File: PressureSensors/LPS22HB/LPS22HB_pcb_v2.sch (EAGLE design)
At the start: 6 parts

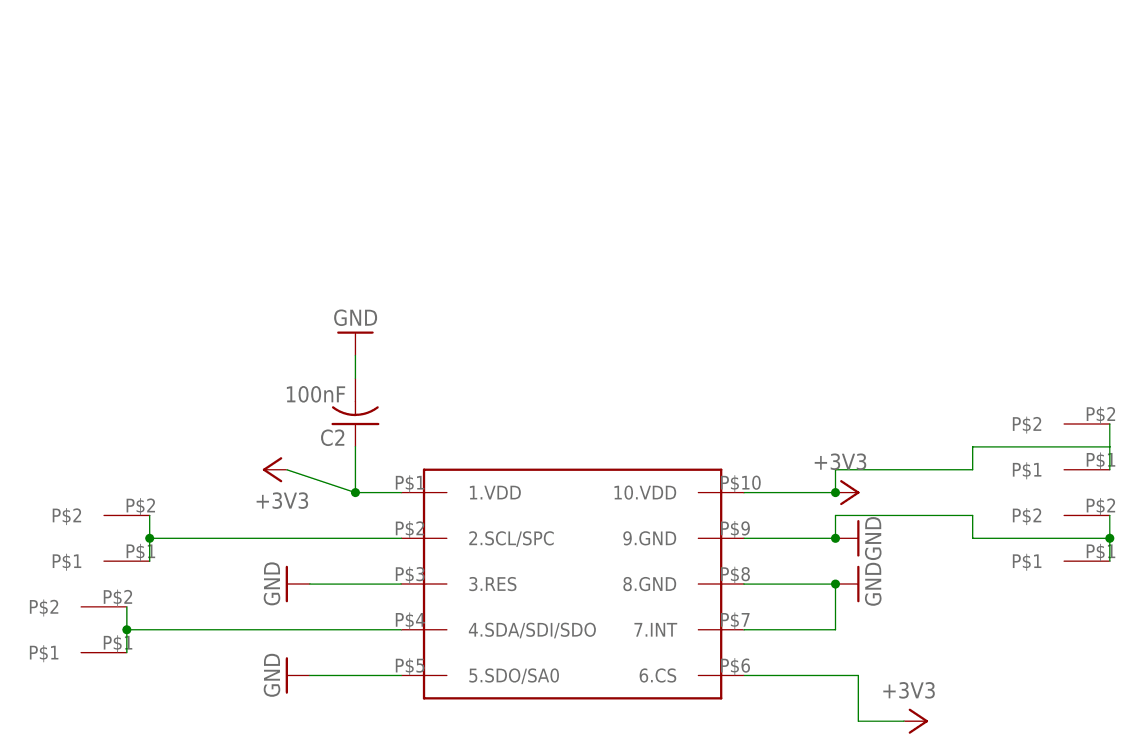
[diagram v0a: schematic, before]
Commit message: overdue changes before messing with plotPSTHStim
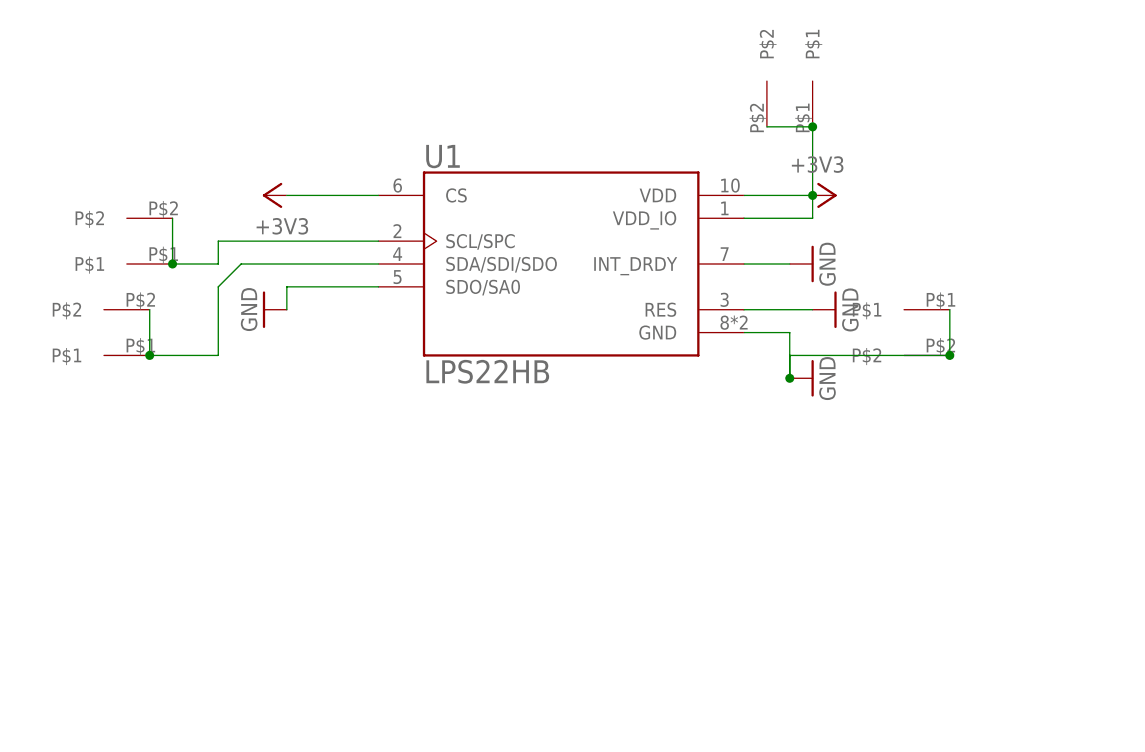
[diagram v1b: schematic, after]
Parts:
- removed C2: 100nF, resistor:C-USC0402
- removed U$3, U$4, U$5: WIREPAD_PADWIREPAD_0,6/0,4_PAD, Sombeck_lib:WIREPAD_PADWIREPAD_0,6/0,4_PAD
- added U$6, U$7: WIREPAD_PADWIREPAD_0,6/0,4_PAD, Sombeck_lib:WIREPAD_PADWIREPAD_0,6/0,4_PAD
- added U1: LPS22HB, LPS22HB:LPS22HB
- U$1: value LPS22HB_HLGA -> WIREPAD_PADWIREPAD_0,6/0,4_PAD; device Sombeck_lib:LPS22HB_HLGA -> Sombeck_lib:WIREPAD_PADWIREPAD_0,6/0,4_PAD
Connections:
- removed net N$1: U$1.2.SCL/SPC, U$2.P$1, U$2.P$2
- removed net N$4: U$1.4.SDA/SDI/SDO, U$3.P$1, U$3.P$2
- new net N$2: U$6.P$1, U$6.P$2, U1.SCL/SPC
- new net N$3: U$7.P$1, U$7.P$2, U1.SDA/SDI/SDO
- net +3V3: now also U$1.P$1, U$1.P$2, U1.CS, U1.VDD, U1.VDD_IO; no longer C2.1, U$1.1.VDD, U$1.10.VDD, U$1.6.CS, U$5.P$1, U$5.P$2
- net GND: now also U$2.P$1, U$2.P$2, U1.GND, U1.INT_DRDY, U1.RES, U1.SDO/SA0; no longer C2.2, U$1.3.RES, U$1.5.SDO/SA0, U$1.7.INT, U$1.8.GND, U$1.9.GND, U$4.P$1, U$4.P$2
